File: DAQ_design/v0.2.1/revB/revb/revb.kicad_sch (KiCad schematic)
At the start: 19 parts, among them Q1 BC549, Q2 IRF9540N, Q3 IRF540N, Q4 BC549, Q5 IRF9540N, Q6 IRF540N, U1 ADS1115IDGS

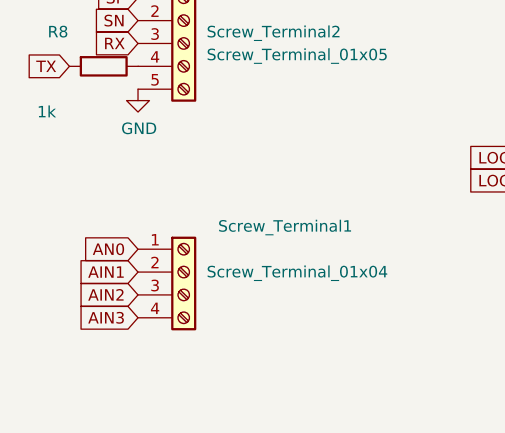
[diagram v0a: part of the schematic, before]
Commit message: attempted fixes
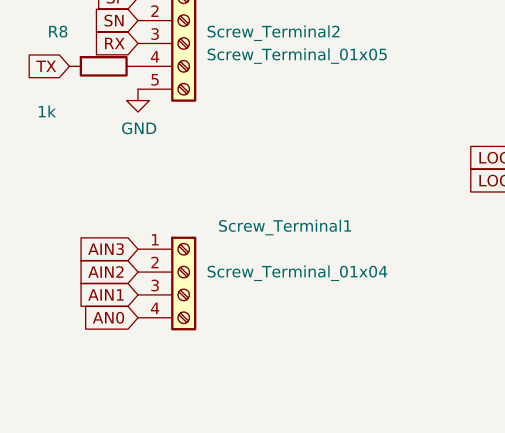
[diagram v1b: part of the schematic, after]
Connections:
- net AIN1: now also Screw_Terminal1.3 (Pin_3); no longer Screw_Terminal1.2 (Pin_2)
- net AIN2: now also Screw_Terminal1.2 (Pin_2); no longer Screw_Terminal1.3 (Pin_3)
- net AIN3: now also Screw_Terminal1.1 (Pin_1); no longer Screw_Terminal1.4 (Pin_4)
- net AN0: now also Screw_Terminal1.4 (Pin_4); no longer Screw_Terminal1.1 (Pin_1)
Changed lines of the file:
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@@
     )
   )
-  (global_label "AN0" (shape input) (at 57.15 152.4 180)
+  (global_label "AN0" (shape input) (at 57.15 160.02 180)
     (effects (font (size 1.27 1.27)) (justify right))
-    (property "Intersheetrefs" "${INTERSHEET_REFS}" (at 57.15 152.4 0)
+    (property "Intersheetrefs" "${INTERSHEET_REFS}" (at 57.15 160.02 0)
       (effects (font (size 1.27 1.27)) hide)
     )
@@
     )
   )
-  (global_label "AIN3" (shape input) (at 57.15 160.02 180)
+  (global_label "AIN3" (shape input) (at 57.15 152.4 180)
     (effects (font (size 1.27 1.27)) (justify right))
-    (property "Intersheetrefs" "${INTERSHEET_REFS}" (at 57.15 160.02 0)
+    (property "Intersheetrefs" "${INTERSHEET_REFS}" (at 57.15 152.4 0)
       (effects (font (size 1.27 1.27)) hide)
     )
@@
     )
   )
-  (global_label "AIN2" (shape input) (at 57.15 157.48 180)
+  (global_label "AIN2" (shape input) (at 57.15 154.94 180)
     (effects (font (size 1.27 1.27)) (justify right))
-    (property "Intersheetrefs" "${INTERSHEET_REFS}" (at 57.15 157.48 0)
+    (property "Intersheetrefs" "${INTERSHEET_REFS}" (at 57.15 154.94 0)
       (effects (font (size 1.27 1.27)) hide)
     )
@@
     )
   )
-  (global_label "AIN1" (shape input) (at 57.15 154.94 180)
+  (global_label "AIN1" (shape input) (at 57.15 157.48 180)
     (effects (font (size 1.27 1.27)) (justify right))
-    (property "Intersheetrefs" "${INTERSHEET_REFS}" (at 57.15 154.94 0)
+    (property "Intersheetrefs" "${INTERSHEET_REFS}" (at 57.15 157.48 0)
       (effects (font (size 1.27 1.27)) hide)
     )
